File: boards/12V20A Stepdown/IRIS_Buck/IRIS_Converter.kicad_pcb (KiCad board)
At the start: 4 copper layers, 50 x 40 mm, 27 parts, among them J1 TB005-762-02BE, J2 TB005-762-02BE, Q1 CSD17571Q2, Q2 CSD16340Q3, U1 LM25145RGYR

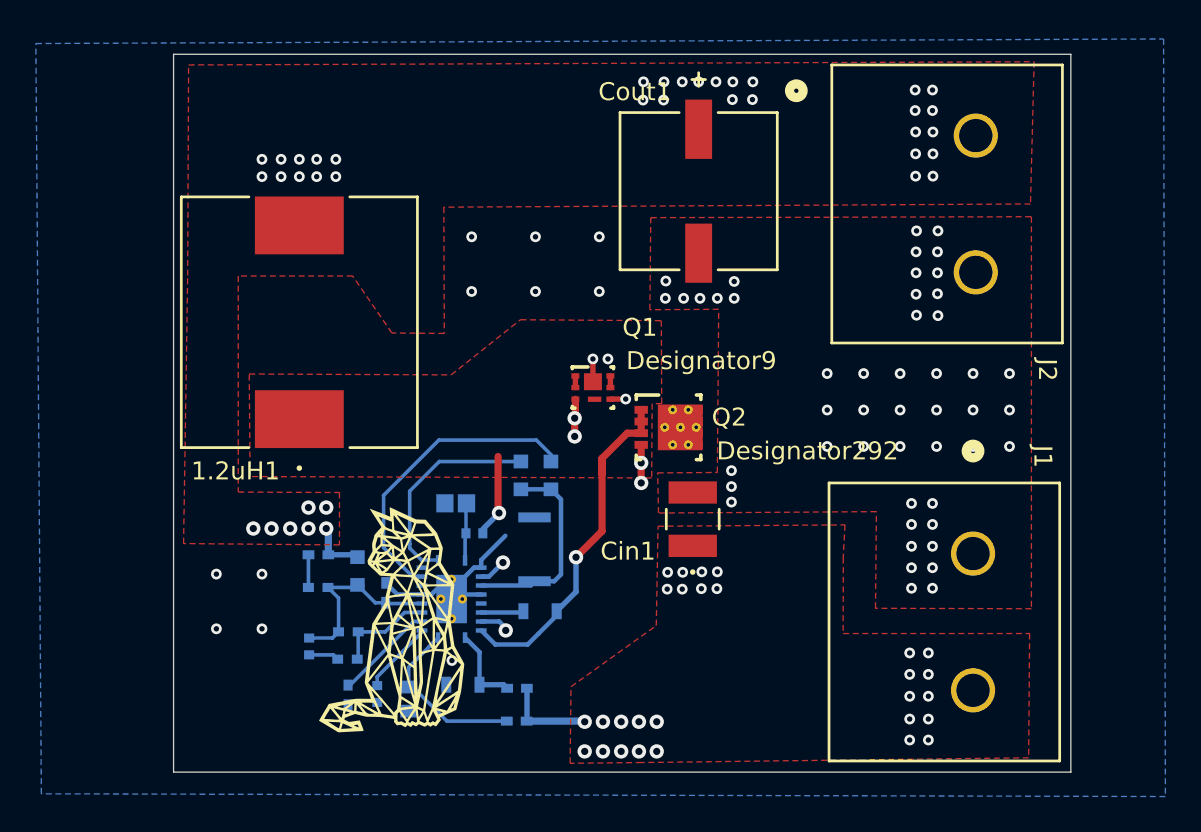
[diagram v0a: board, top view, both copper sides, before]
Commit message: Added mounting holes and generated manu files
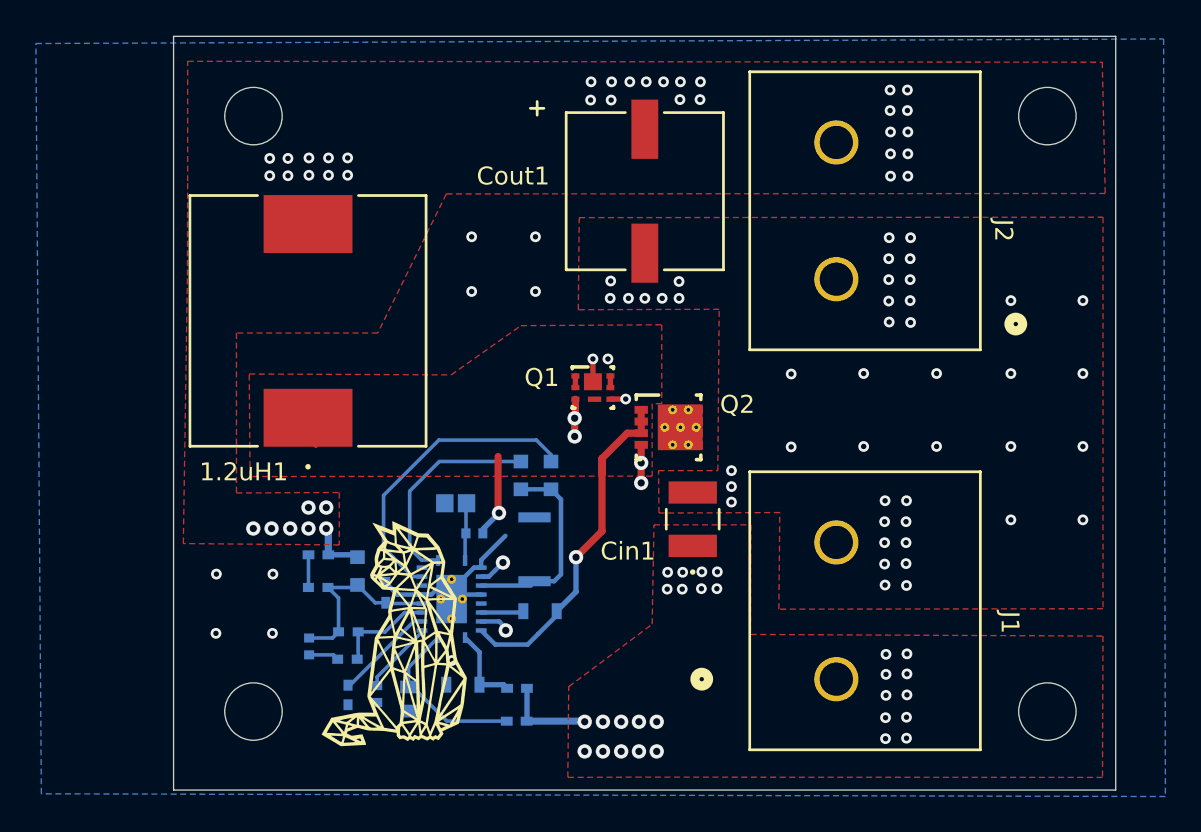
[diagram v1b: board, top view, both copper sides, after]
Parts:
- added REF**: MountingHole_3.2mm_M3, MountingHole:MountingHole_3.2mm_M3, F.Cu at (124.0, 42.6)
- added REF**: MountingHole_3.2mm_M3, MountingHole:MountingHole_3.2mm_M3, F.Cu at (124.0, 75.7)
- added REF**: MountingHole_3.2mm_M3, MountingHole:MountingHole_3.2mm_M3, F.Cu at (79.8, 42.6)
- added REF**: MountingHole_3.2mm_M3, MountingHole:MountingHole_3.2mm_M3, F.Cu at (79.8, 75.7)
- moved J2 11.2 mm to (112.3, 51.6), turned to 90 degrees
- moved J1 10.3 mm to (112.3, 73.9), turned to 90 degrees
- moved Cout1 3.00 mm to (101.6, 46.7)
- moved 1.2uH1 0.49 mm to (82.8, 54.0)
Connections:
- J1 pad 1: GND -> /Vin
- J1 pad 2: /Vin -> GND
- J2 pad 1: /Vout -> GND
- J2 pad 2: GND -> /Vout
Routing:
- net GND: vias 62 -> 56
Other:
- board size 50 x 40 mm -> 52.5 x 42 mm
